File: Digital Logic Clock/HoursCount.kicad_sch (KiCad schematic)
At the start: 19 parts, among them U1 4081

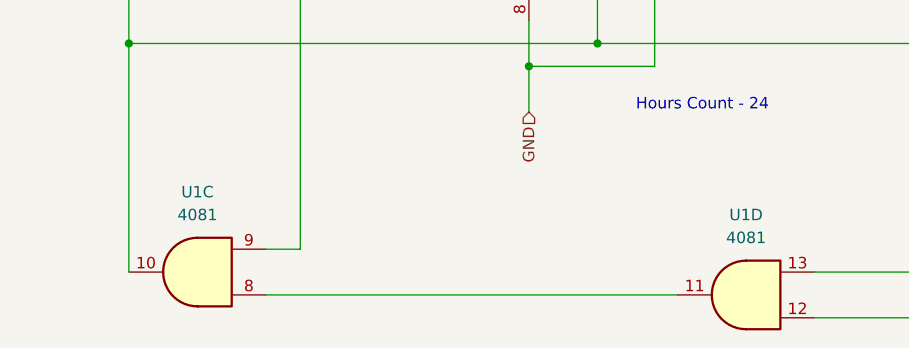
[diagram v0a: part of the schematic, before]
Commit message: Clock Project
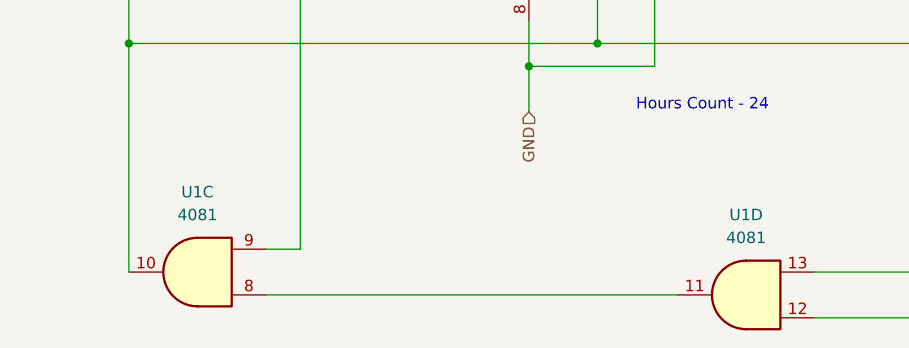
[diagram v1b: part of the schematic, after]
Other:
- company: (none) -> Akbar Q
- title: (none) -> Hours Counter
